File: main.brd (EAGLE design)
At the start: 50.8 x 40.6 mm, 30 parts

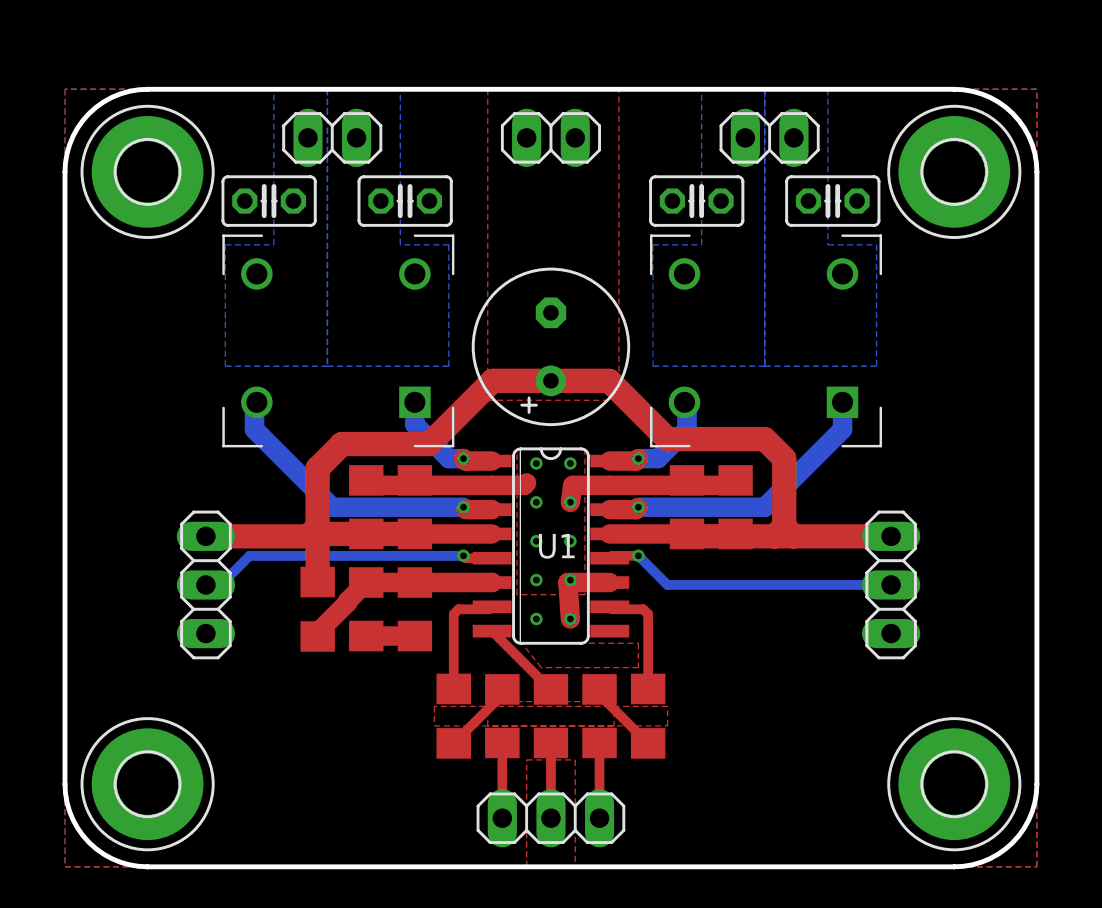
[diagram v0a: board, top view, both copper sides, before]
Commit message: New board design
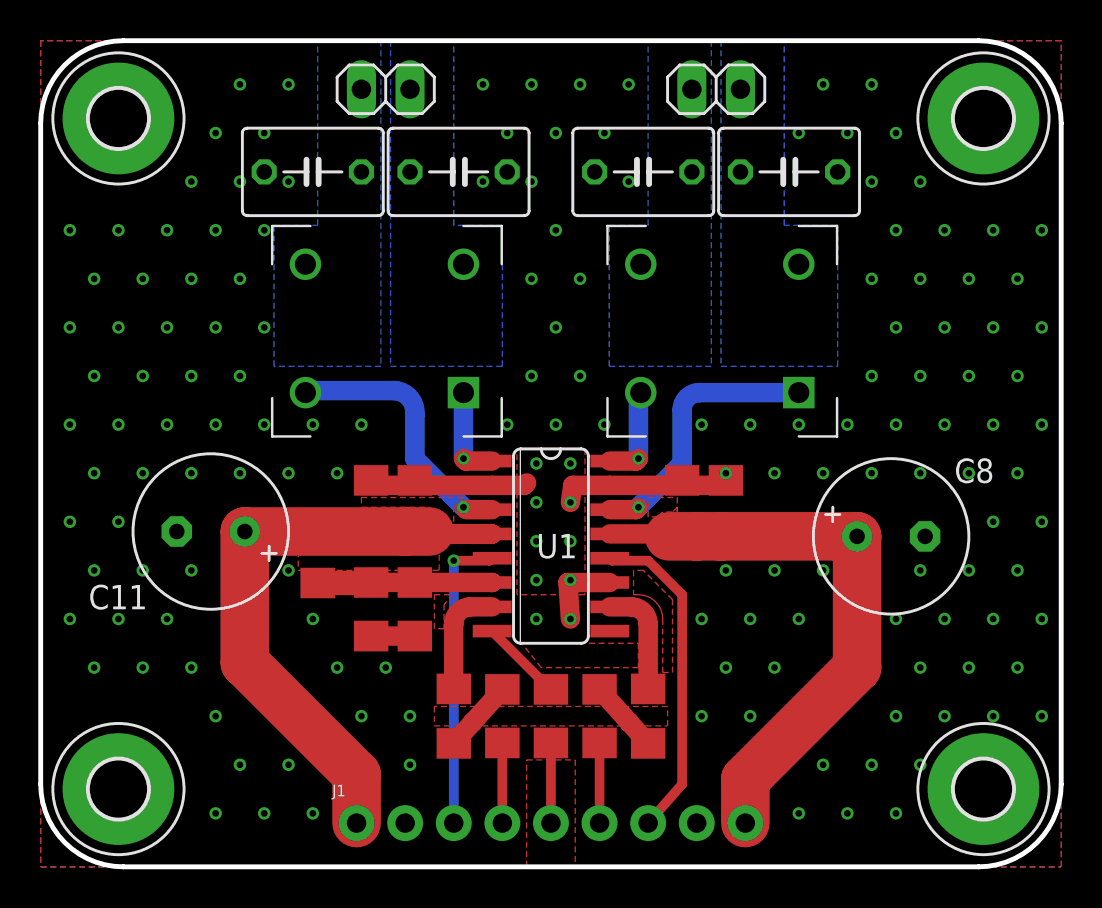
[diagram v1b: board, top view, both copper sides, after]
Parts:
- removed AUDIO_IN, MUTE, SHDN: (no value), pinhead:1X03
- removed VDD: (no value), pinhead:1X02
- added C11: (no value), rcl:E3,5-8
- added J1: (no value), SparkFun-Connectors:1X09_NO_SILK
- C12, C13, C14, C15: device rcl:C025-025X050 -> rcl:C050-045X075
- H1, H2, H3, H4: value MOUNT-PAD-ROUND3.2 -> MOUNT-PAD-ROUND3.0; device holes:3,2-PAD -> holes:3,0-PAD
- moved C8 20.4 mm to (43.2, 27.4), turned to 0 degrees
- moved OUT_L 3.78 mm to (16.8, 50.8)
- moved OUT_R 3.78 mm to (34.0, 50.8)
- moved C14 3.18 mm to (30.2, 46.5)
- moved H2 3.18 mm to (48.0, 49.3)
- moved H3 3.18 mm to (2.79, 49.3)
- moved C13 3.18 mm to (20.6, 46.5)
- moved R3 2.79 mm to (13.2, 26.4)
- moved C12 2.75 mm to (13.0, 46.5)
- moved C15 2.75 mm to (37.8, 46.5)
- moved LEFT_COIL 2.59 mm to (20.8, 41.7)
- moved RIGHT_COIL 2.34 mm to (38.4, 41.7)
- moved H1 1.55 mm to (48.0, 14.2)
- moved H4 1.55 mm to (2.79, 14.2)
- moved C10 0.51 mm to (34.5, 29.0)
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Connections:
- removed net !MUTE: MUTE.2, U1.5
- removed net !SHND: SHDN.2, U1.12
- new net MUTE: J1.3, U1.5
- new net SHDN: J1.7, U1.12
- net GND: now also C11.-, H1.B3,0, H2.B3,0, H3.B3,0, H4.B3,0, J1.2, J1.5, J1.8; no longer AUDIO_IN.2, MUTE.3, SHDN.3, VDD.1
- net N$3: now also J1.4; no longer AUDIO_IN.1
- net N$5: now also J1.6; no longer AUDIO_IN.3
- net VDD: now also C11.+, J1.1, J1.9; no longer MUTE.1, SHDN.1, VDD.2
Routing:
- net SHDN: track 0.00 -> 17.2 mm
- net MUTE: track 0.00 -> 15.8 mm, vias 0 -> 1
- net !MUTE: track 15.6 -> 0.00 mm, vias 1 -> 0
- net !SHND: track 15.4 -> 0.00 mm, vias 1 -> 0
- net OUT_L-: track 15.6 -> 13.8 mm
- net OUT_R-: track 16.8 -> 15.6 mm
- net OUT_R+: track 6.20 -> 5.05 mm
- net AVDD: track 10.5 -> 9.42 mm
- net OUT_L+: track 5.99 -> 5.00 mm
- net VDD: track 74.6 -> 73.8 mm
- net GND: track 29.2 -> 28.9 mm, vias 10 -> 161
- added copper zone on layer 1, net N$13
- added copper zone on layer 1, net N$14
- added copper zone on layer 1, net N$15
- added copper zone on layer 1, net N$16
- added copper zone on layer 1, net N$17
- removed copper zone on layer 1, net N$9
- removed copper zone on layer 1, net VDD
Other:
- board size 50.8 x 40.6 mm -> 53.3 x 43.2 mm
- board text added: "COMMON"
- board text added: "GND"
- board text added: "LEFT"
- board text added: "LEFT+"
- board text added: "LEFT−"
- board text added: "MUTE"
- board text added: "RIGHT"
- board text added: "RIGHT+"
- board text added: "RIGHT−"
- board text added: "SHDN"
- board text added: "VCC"
- board text added: "© 2017 FATIH YILMAZ LICENSED UNDER THE TAPR OHL V 1.0"
